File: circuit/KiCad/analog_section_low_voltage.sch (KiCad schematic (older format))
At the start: 40 parts, among them J6 Screw_Terminal_01x09, J7 Screw_Terminal_01x09, U11 LM7332, U12 CPC1114N, U13 CPC1114N

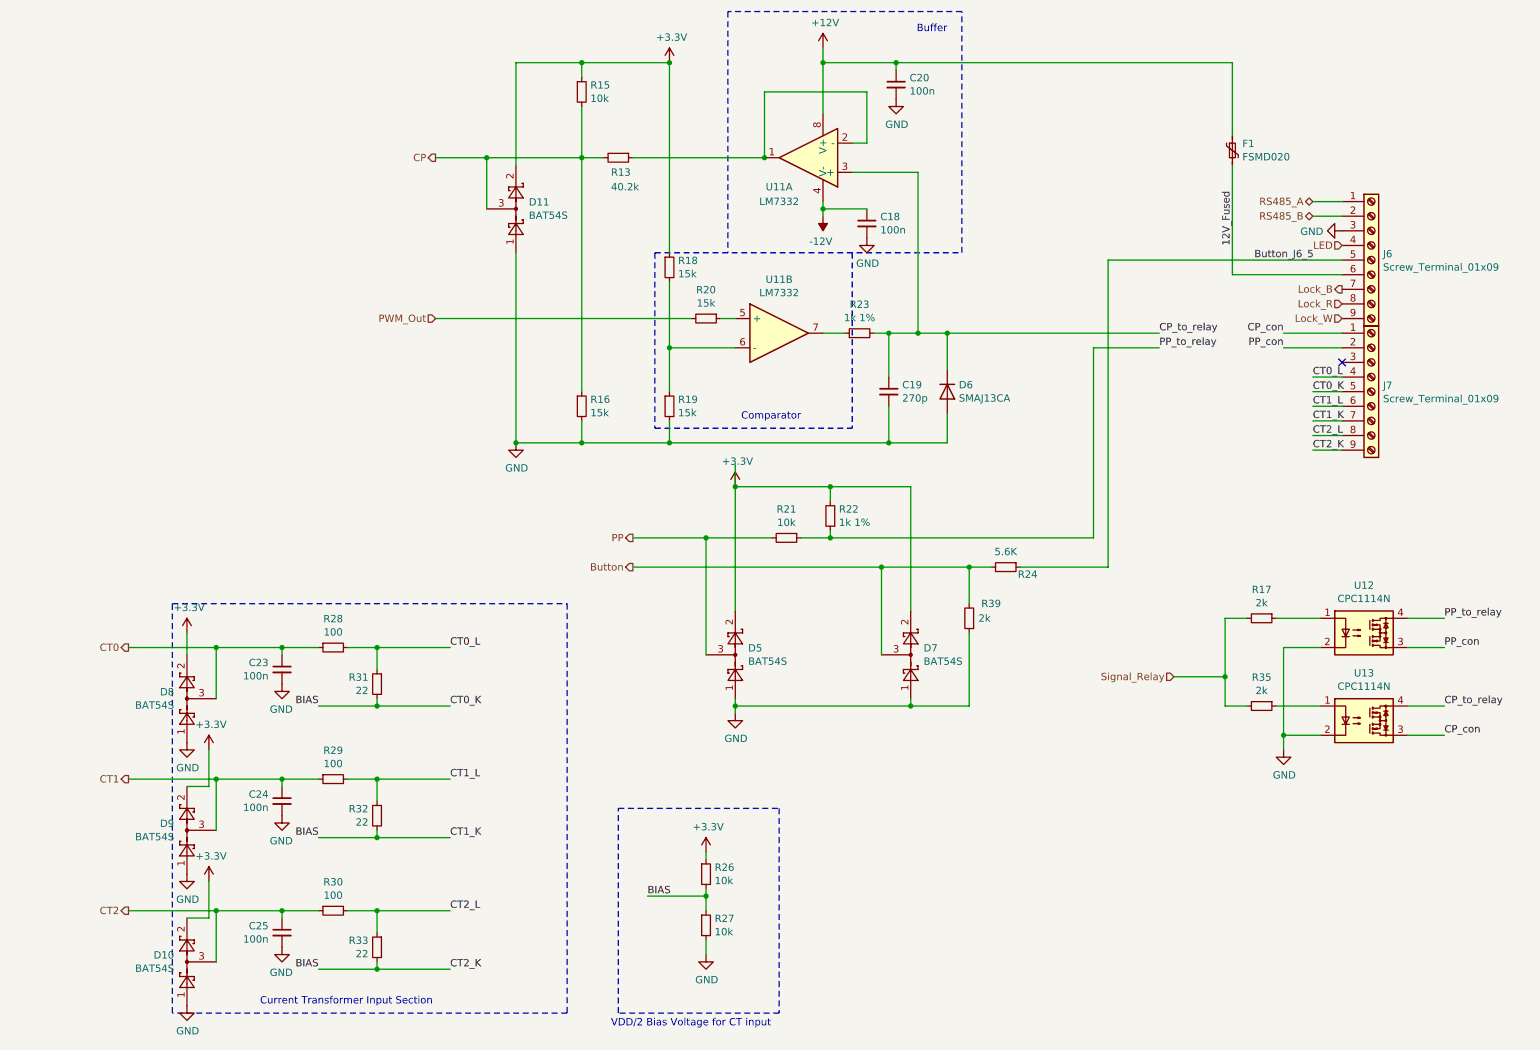
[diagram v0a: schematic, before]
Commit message: qe
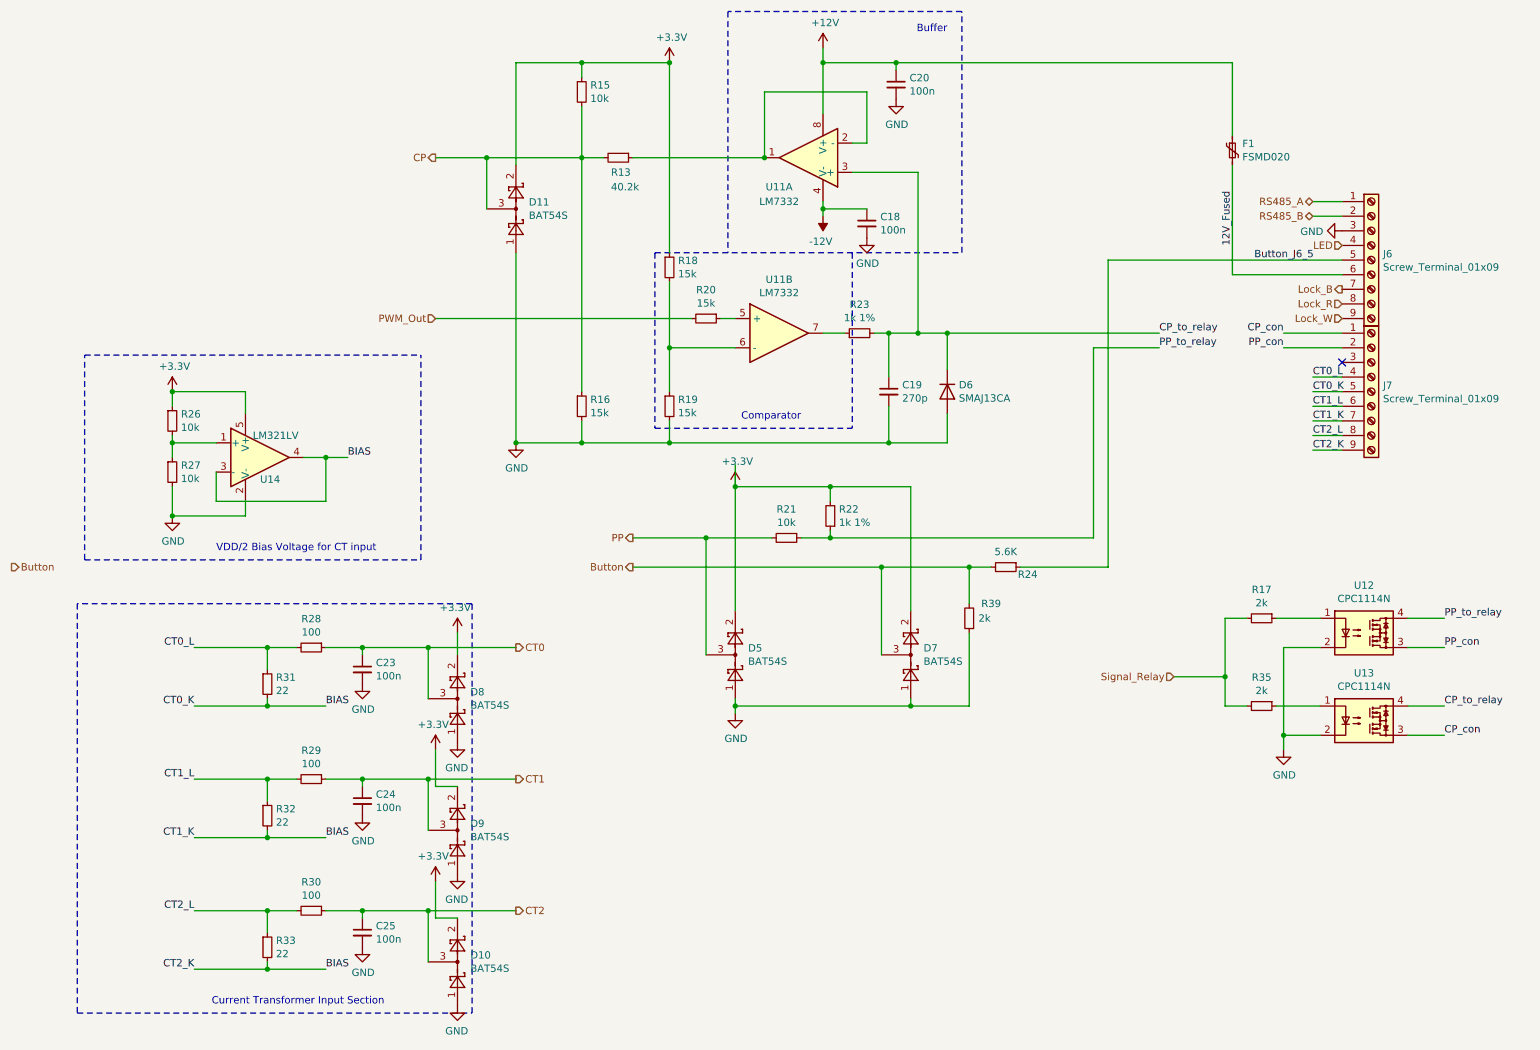
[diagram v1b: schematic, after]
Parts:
- added U14: LM321LV, Package_TO_SOT_SMD:SOT-23-5, symbol Amplifier_Operational:LM321
- R39: footprint Resistor_SMD:R_0603_1608Metric_Pad0.98x0.95mm_HandSolder -> Resistor_SMD:R_0603_1608Metric_Pad1.05x0.95mm_HandSolder
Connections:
- net +3V3: now also U14.5 (V+)
- net BIAS: now also U14.3 (-), U14.4; no longer R26.2, R27.1
- net GND: now also U14.2 (V-)
- new net: R26.2, R27.1, U14.1 (+)
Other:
- moved on the sheet: C23, C24, C25, D10, D8, D9, R26, R27, R28, R29, R30, R31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
